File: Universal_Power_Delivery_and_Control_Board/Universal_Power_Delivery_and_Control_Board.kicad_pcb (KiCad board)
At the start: 4 copper layers, 99.5 x 99.5 mm, 160 parts, among them CN1 B03B-XASK-1-A(LF)(SN), CN2 B03B-XASK-1-A(LF)(SN), CN3 B03B-XASK-1-A(LF)(SN), CN4 B03B-XASK-1-A(LF)(SN), Q1 PMZ600UNEYL, Q2 PMZ600UNEYL, SW2 TS1102-TD35HBM, U1 TPS259470LRPWR, U10 SN74LVC1G17DCKR, U11 SN74LVC1G17DCKR, U12 SN74LVC1G17DCKR, U13 SN74LVC1G17DCKR, U14 SN74LVC1G17DCKR, U15 SN74LVC541APWR_C113281, U16 SN74LVC541APWR_C113281, U17 SN74LVC1G17DCKR, U18 LM66200DRLR, U19 TF-0803-0, U2 CH224Q_C46061833, U20 TCA9555PWR, U21 TPS22919DCK, U22 HC-PM254-8.5H-2X4PW-02A, U3 USBLC6-2SC6, U4 ESD2CAN24-ES, U5 S2B-ZR (LF)(SN), U6 USBLC6-2SC6, U7 TPS54202DDC, U8 TPS51385RJNR, U9 TPS24751RUVR

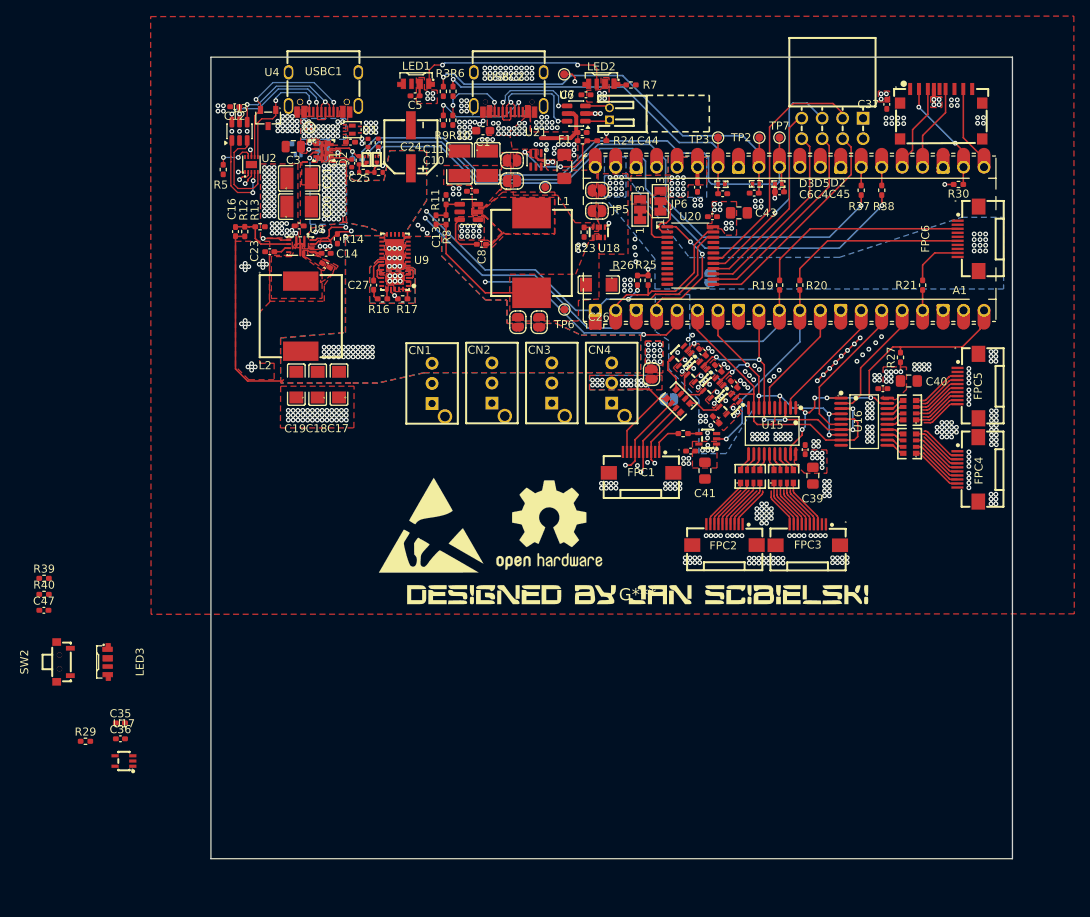
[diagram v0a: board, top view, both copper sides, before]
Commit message: Fished layout for now, need to add some components for optional functionality.
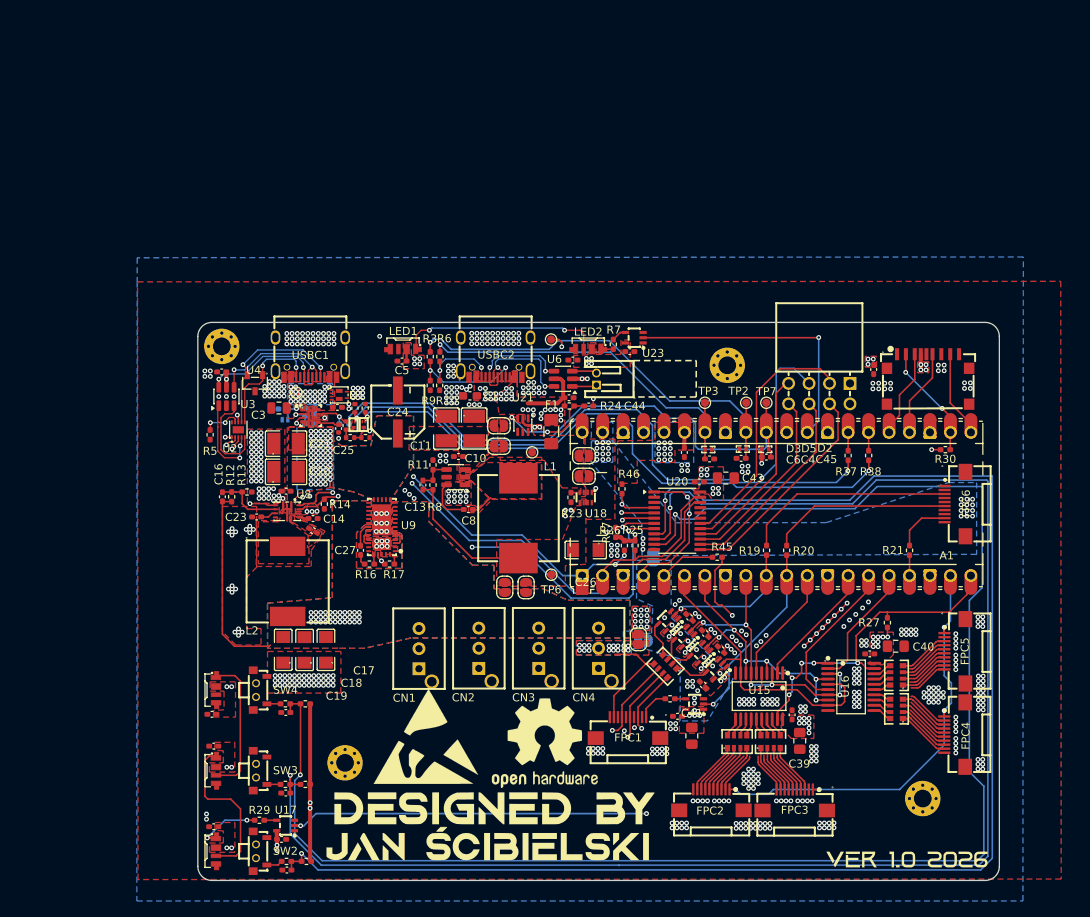
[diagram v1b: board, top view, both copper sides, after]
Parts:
- removed the G*** at (155.1, 104.9)
- removed JP5, JP6: SolderJumper_3_Bridged12, Jumper:SolderJumper-3_P1.3mm_Bridged12_Pad1.0x1.5mm_NumberLabels
- added C48: 100nF, Capacitor_SMD:C_0402_1005Metric_Pad0.74x0.62mm_HandSolder, F.Cu at (102.5, 123.7)
- added C49: 100nF, Capacitor_SMD:C_0402_1005Metric_Pad0.74x0.62mm_HandSolder, F.Cu at (111.4, 129.6)
- added C50: 100nF, Capacitor_SMD:C_0402_1005Metric_Pad0.74x0.62mm_HandSolder, F.Cu at (102.3, 119.8)
- added C51: 100nF, Capacitor_SMD:C_0402_1005Metric_Pad0.74x0.62mm_HandSolder, F.Cu at (111.4, 119.5)
- added C52: 100nF, Capacitor_SMD:C_0402_1005Metric_Pad0.74x0.62mm_HandSolder, F.Cu at (154.2, 74.8)
- added G***: LOGO, LOGO, F.Cu at (188.6, 137.8)
- added G***: LOGO, LOGO, F.Cu at (137.5, 131.4)
- added G***: LOGO, LOGO, F.Cu at (136.5, 136.2)
- added H1: MountingHole_Pad, MountingHole:MountingHole_2.2mm_M2_Pad_Via, F.Cu at (103.5, 74.1)
- added H2: MountingHole_Pad, MountingHole:MountingHole_2.2mm_M2_Pad_Via, F.Cu at (166.2, 76.5)
- added H3: MountingHole_Pad, MountingHole:MountingHole_2.2mm_M2_Pad_Via, F.Cu at (118.8, 125.8)
- added H4: MountingHole_Pad, MountingHole:MountingHole_2.2mm_M2_Pad_Via, F.Cu at (190.5, 130.2)
- added LED4: SK6812SIDE-A_C5378721, lcsc_footprints:C5378721_LED-SMD_4P-L4_0-W1_6-L, F.Cu at (102.8, 126.8)
- added LED5: SK6812SIDE-A_C5378721, lcsc_footprints:C5378721_LED-SMD_4P-L4_0-W1_6-L, F.Cu at (102.8, 116.8)
- added R41: 100K, Resistor_SMD:R_0402_1005Metric_Pad0.72x0.64mm_HandSolder, F.Cu at (113.9, 128.5)
- added R42: 10K, Resistor_SMD:R_0402_1005Metric_Pad0.72x0.64mm_HandSolder, F.Cu at (111.4, 128.5)
- added R43: 100K, Resistor_SMD:R_0402_1005Metric_Pad0.72x0.64mm_HandSolder, F.Cu at (113.9, 118.5)
- added R44: 10K, Resistor_SMD:R_0402_1005Metric_Pad0.72x0.64mm_HandSolder, F.Cu at (111.4, 118.5)
- added R45: 33R, Resistor_SMD:R_0402_1005Metric_Pad0.72x0.64mm_HandSolder, F.Cu at (165.0, 100.3)
- added R46: 10K, Resistor_SMD:R_0402_1005Metric_Pad0.72x0.64mm_HandSolder, F.Cu at (153.2, 91.8)
- added R47: 10K, Resistor_SMD:R_0402_1005Metric_Pad0.72x0.64mm_HandSolder, F.Cu at (152.4, 97.2)
- added SW3: TS1102-TD35HBM, lcsc_footprints:C36936640_SW-SMD_TS1102-TD35HBM, F.Cu at (108.2, 126.8)
- added SW4: TS1102-TD35HBM, lcsc_footprints:C36936640_SW-SMD_TS1102-TD35HBM, F.Cu at (108.2, 116.8)
- added U23: SN74LVC1G17DCKR, lcsc_footprints:C10425_SC-70-5_L2_1-W1_3-P0_65-LS2_1-BR, F.Cu at (154.7, 73.0)
- moved R39 47.9 mm to (114.0, 138.0), turned to 180 degrees
- moved R40 44.8 mm to (111.5, 138.0)
- moved C47 44.2 mm to (111.6, 139.1)
- moved JP3 35.4 mm to (157.1, 100.2), turned to 90 degrees
- moved SW2 33.9 mm to (108.2, 136.8)
- moved C17 33.0 mm to (116.4, 111.8)
- moved C19 33.0 mm to (111.1, 111.8)
- moved C32 33.0 mm to (160.1, 120.0)
- moved C34 33.0 mm to (183.9, 112.3)
- moved FPC2 33.0 mm to (164.3, 130.4)
- moved JP1 33.0 mm to (138.6, 104.0)
- moved JP2 33.0 mm to (141.3, 104.0)
- moved L2 33.0 mm to (111.7, 103.3)
- moved RN5 33.0 mm to (187.3, 114.9)
- moved U10 33.0 mm to (164.9, 114.2)
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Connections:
- net /Power_Output/5V_O1 renamed /Digital_Signal_Output/CLK
- net /Power_Output/5V_O2 renamed /Digital_Signal_Output/LE
- net /Power_Output/5V_O3 renamed /Digital_Signal_Output/OE
- A1 pad 29: /PD_Section/IND_LED_DIN -> /UI_Section/IND_LED_DIN
- A1 pad 5: unconnected-(A1-GPIO3-Pad5) -> Net-(A1-GPIO3)
- C36 pad 1: Net-(U17-VCC) -> +5V_VSYS
- C36 pad 2: Net-(U17-GND) -> GND
- C47 pad 2: Net-(C47-Pad2) -> /P05
- LED1 pad 3: /PD_Section/IND_LED_DOUT -> unconnected-(LED1-DOUT-Pad3)
- LED3 pad 3: unconnected-(LED3-DOUT-Pad3) -> Net-(LED3-DOUT)
- R14 pad 1: /Power_Output/EN_TPS51385 -> /P02
- R17 pad 1: /P00 -> /P04
- R39 pad 2: Net-(C47-Pad2) -> /P05
- R40 pad 2: Net-(C47-Pad2) -> /P05
- R7 pad 1: /PD_Section/IND_LED_DIN -> Net-(U23-Y)
- U1 pad 3: /PD_Section/PG_eFUSE -> /P00
- U17 pad 2: unconnected-(U17-A-Pad2) -> /Button_LED_DIN
- U17 pad 3: Net-(U17-GND) -> GND
- U17 pad 5: Net-(U17-VCC) -> +5V_VSYS
- U20 pad 10: unconnected-(U20-P06-Pad10) -> /P06
- U20 pad 11: unconnected-(U20-P07-Pad11) -> /P07
- U20 pad 2: Net-(JP6-C) -> GND
- U20 pad 3: Net-(JP5-C) -> GND
- U8 pad 11: /Power_Output/EN_TPS51385 -> /P02
- U8 pad 12: /Power_Output/MODE_TPS51385 -> /P01
- U8 pad 3: /Power_Output/PG_TPS51385 -> /P03
- U9 pad 33: /P00 -> /P04
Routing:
- net /P07: track 0.00 -> 198.7 mm, vias 0 -> 2
- net /P06: track 0.00 -> 194.5 mm, vias 0 -> 2
- net /P05: track 0.00 -> 186.8 mm, vias 0 -> 2
- net +3V3: track 8.29 -> 102.7 mm, vias 57 -> 60
- net /Button_LED_DIN: track 0.00 -> 82.1 mm, vias 0 -> 3
- net /P03: track 0.00 -> 57.7 mm, vias 0 -> 4
- net /PD_Section/PG_eFUSE: track 55.2 -> 0.00 mm, vias 2 -> 0
- net /Digital_Signal_Output/HIGH_CURRENT_EN: track 0.00 -> 53.8 mm, vias 0 -> 4
- net /Power_Output/PG_TPS51385: track 52.7 -> 0.00 mm, vias 4 -> 0
- net /P01: track 0.00 -> 48.5 mm, vias 0 -> 3
- net /P02: track 0.00 -> 47.9 mm, vias 0 -> 3
- net /P04: track 0.00 -> 47.7 mm, vias 0 -> 3
- net /Power_Output/MODE_TPS51385: track 44.4 -> 0.00 mm, vias 3 -> 0
- net /Power_Output/EN_TPS51385: track 43.8 -> 0.00 mm, vias 3 -> 0
- net /UI_Section/IND_LED_DIN: track 0.00 -> 34.2 mm, vias 0 -> 1
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- added copper zone on B.Cu, net GND
- added copper zone on In2.Cu, net Net-(U21-IN)
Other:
- board size 99.5 x 99.5 mm -> 99.5 x 69.3 mm
